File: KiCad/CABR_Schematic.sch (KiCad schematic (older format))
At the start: 23 parts, among them J1 Screw_Terminal_01x02, J2 0.1\" Header, J3 Program Header, J4 MicroSwitch, J5 Screw_Terminal_01x02, M1 Solenoid, Q1 PBSS4250X, SW1 Fire Mode, SW2 Microswitch, U1 AZ1117-5.0, U2 ATtiny85-20SU

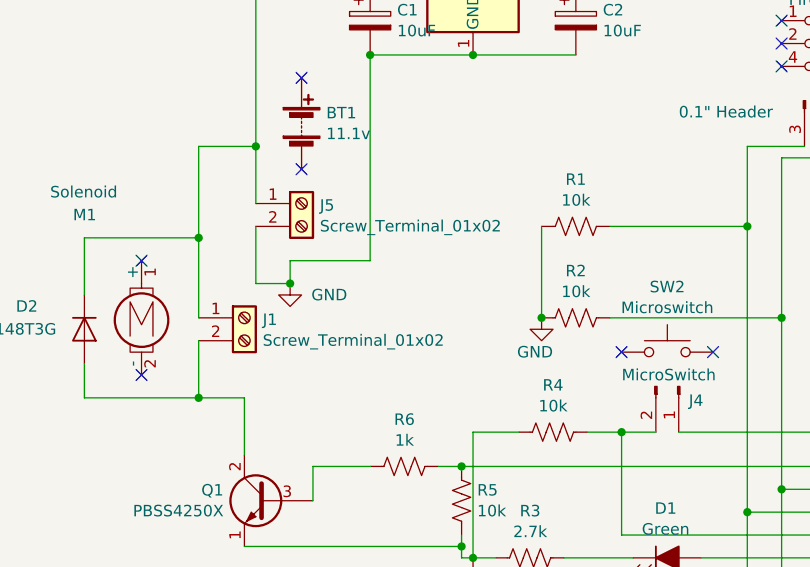
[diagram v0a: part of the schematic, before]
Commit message: redid file structure
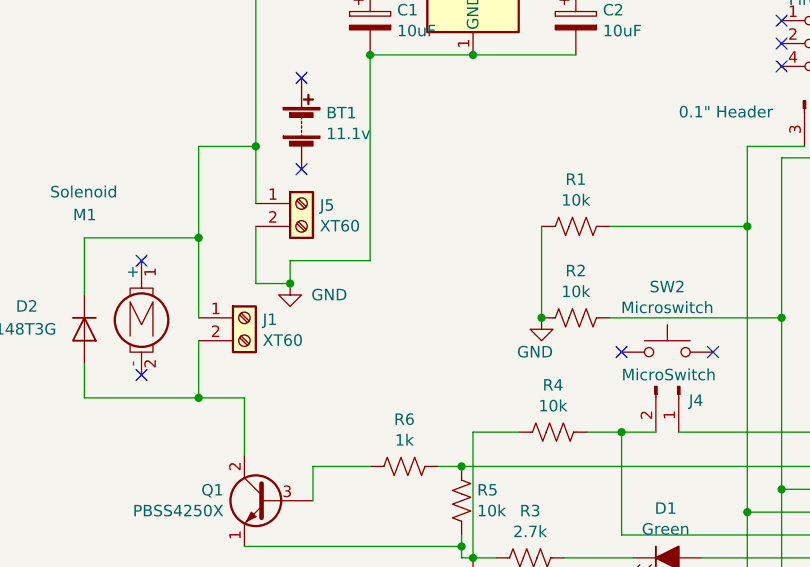
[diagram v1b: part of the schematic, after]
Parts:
- J1, J5: value Screw_Terminal_01x02 -> XT60
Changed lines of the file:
@@
 P 4750 3150
 F 0 "J1" H 4830 3142 50  0000 L CNN
-F 1 "Screw_Terminal_01x02" H 4830 3051 50  0000 L CNN
+F 1 "XT60" H 4830 3051 50  0000 L CNN
 F 2 "XT60:XT60" H 4750 3150 50  0001 C CNN
 F 3 "~" H 4750 3150 50  0001 C CNN
@@
 P 5000 2650
 F 0 "J5" H 5080 2642 50  0000 L CNN
-F 1 "Screw_Terminal_01x02" H 5080 2551 50  0000 L CNN
+F 1 "XT60" H 5080 2551 50  0000 L CNN
 F 2 "XT60:XT60" H 5000 2650 50  0001 C CNN
 F 3 "~" H 5000 2650 50  0001 C CNN
